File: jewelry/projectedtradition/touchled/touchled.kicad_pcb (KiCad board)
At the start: 2 copper layers, 22 x 22 mm, 10 parts, among them J1 Conn_01x01, J2 Conn_01x01, J3 Conn_01x01, J4 Conn_01x01, U1 TPP223-BA6

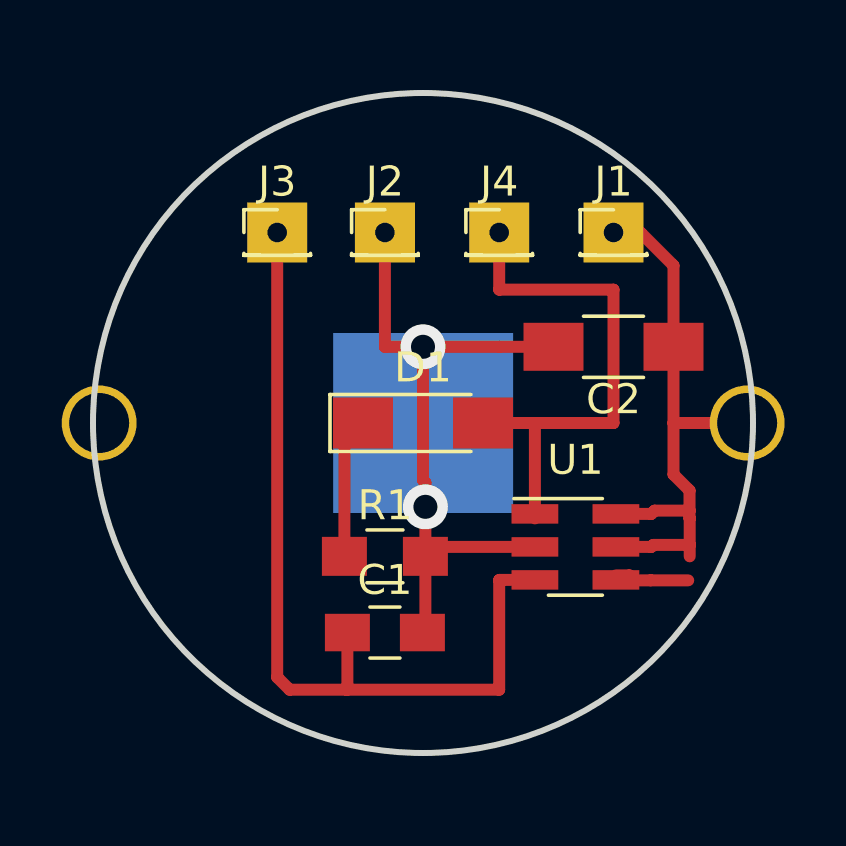
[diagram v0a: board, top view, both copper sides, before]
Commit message: jewelry: Initial layout for touchled
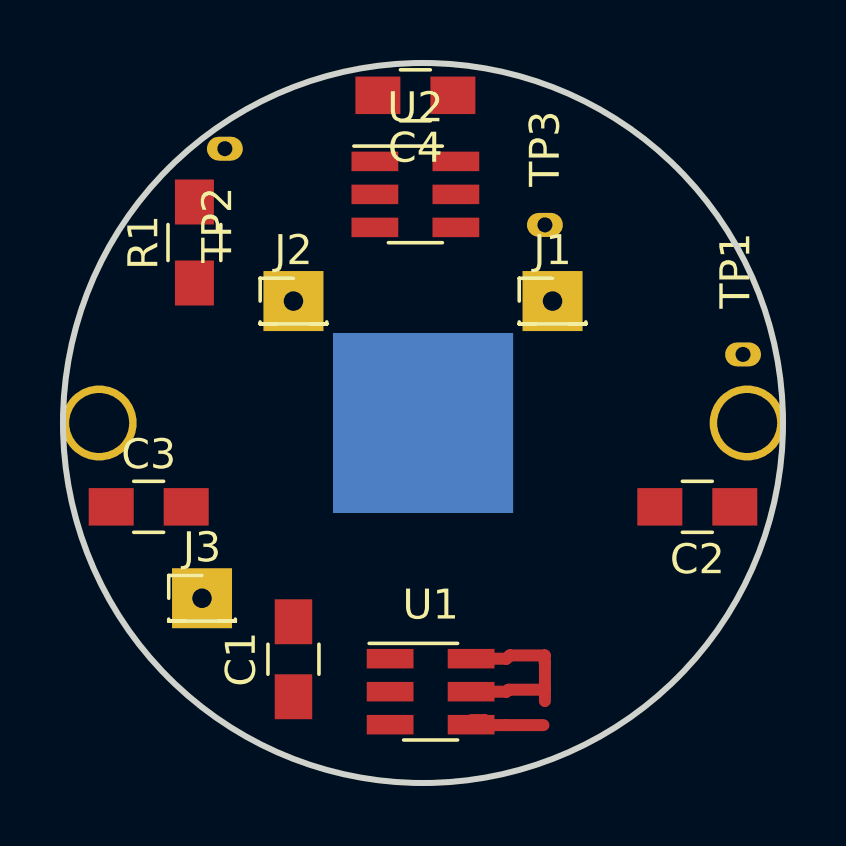
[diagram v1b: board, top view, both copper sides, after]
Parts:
- removed D1: LED, LEDs:LED_1206_HandSoldering
- removed J4: Conn_01x01, Pin_Headers:Pin_Header_Straight_1x01_Pitch1.27mm
- added C3: 1uF, Capacitors_SMD:C_0805_HandSoldering, F.Cu at (-9.14, 2.79)
- added C4: 1uF, Capacitors_SMD:C_0805_HandSoldering, F.Cu at (-0.25, -10.9)
- added TP1: TEST, touchuc:progpin, F.Cu at (10.7, -2.29)
- added TP2: TEST, touchuc:progpin, F.Cu at (-6.60, -9.14)
- added TP3: TEST, touchuc:progpin, F.Cu at (4.06, -6.60)
- added U2: AP3019A, touchled:SOT-223-6-extraspace, F.Cu at (-0.25, -7.62)
- BT1: footprint touchflower:BK-913 -> touchled:BK-913
- C1: value C -> 47pF
- C2: value CP -> 1uF; footprint Capacitors_SMD:C_1206_HandSoldering -> Capacitors_SMD:C_0805_HandSoldering
- R1: value R -> 22R
- U1: footprint touchflower:SOT-223-6-extraspace -> touchled:SOT-223-6-extraspace
- moved J3 12.4 mm to (-7.37, 5.84)
- moved R1 12.2 mm to (-7.62, -6.02), turned to 90 degrees
- moved U1 6.82 mm to (0.25, 8.96)
- moved C2 6.02 mm to (9.14, 2.79)
- moved J2 3.81 mm to (-4.32, -4.06)
- moved C1 3.17 mm to (-4.32, 7.87), turned to 90 degrees
- moved J1 3.06 mm to (4.32, -4.06)
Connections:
- J1 pad 1: VDD -> /LED+
- J2 pad 1: GND -> /LED-
- R1 pad 1: Net-(D1-Pad1) -> /LED-
- U1 pad 1: /out -> touchon
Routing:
- net /sensor: track 29.2 -> 0.00 mm
- net GND: track 23.6 -> 0.00 mm, vias 2 -> 0
- net /out: track 17.7 -> 0.00 mm
- net VDD: track 19.5 -> 6.52 mm
- net Net-(D1-Pad1): track 4.70 -> 0.00 mm
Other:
- board size 22 x 22 mm -> 24 x 24 mm
